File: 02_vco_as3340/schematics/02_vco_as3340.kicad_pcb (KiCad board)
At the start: 2 copper layers, 75 x 100 mm, 89 parts, among them J1 Header 1, J10 SINE OUT, J2 Header 2, J3 SYNC IN, J4 FM IN, J5 PWM CV IN, J6 1V per O IN, J7 SQUARE OUT, J8 SAW OUT, J9 TRI OUT, Q1 BC547C, Q2 BC547C, U1 TL072, U2 AS3340, U3 TL074

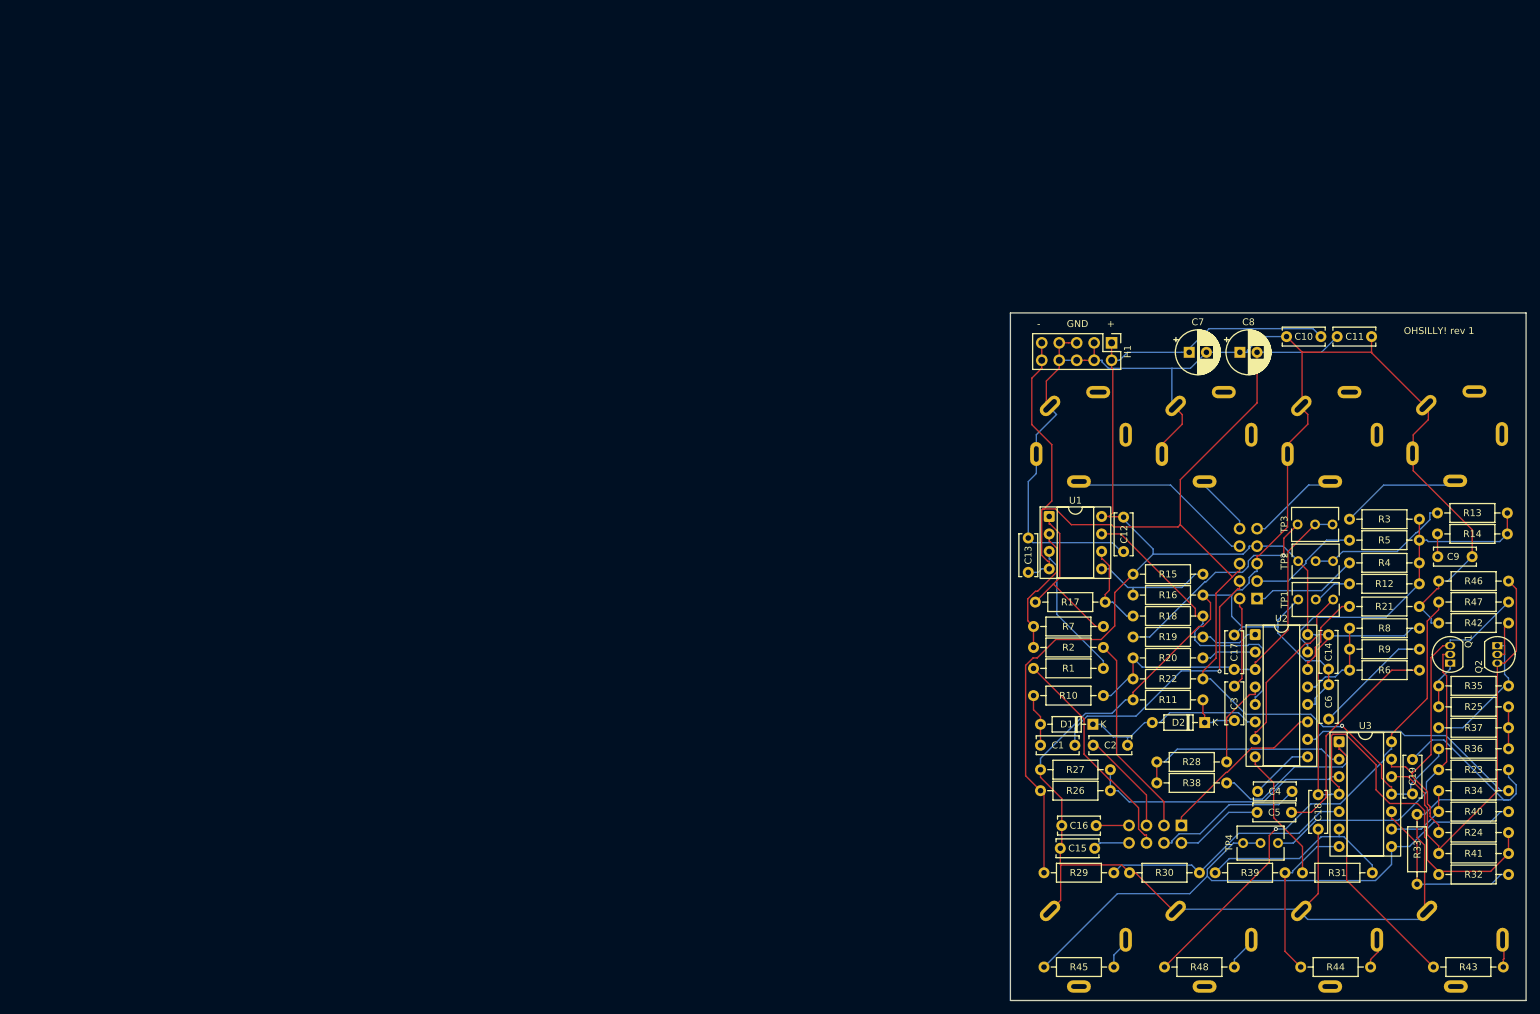
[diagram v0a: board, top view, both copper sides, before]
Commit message: 02 SMD!
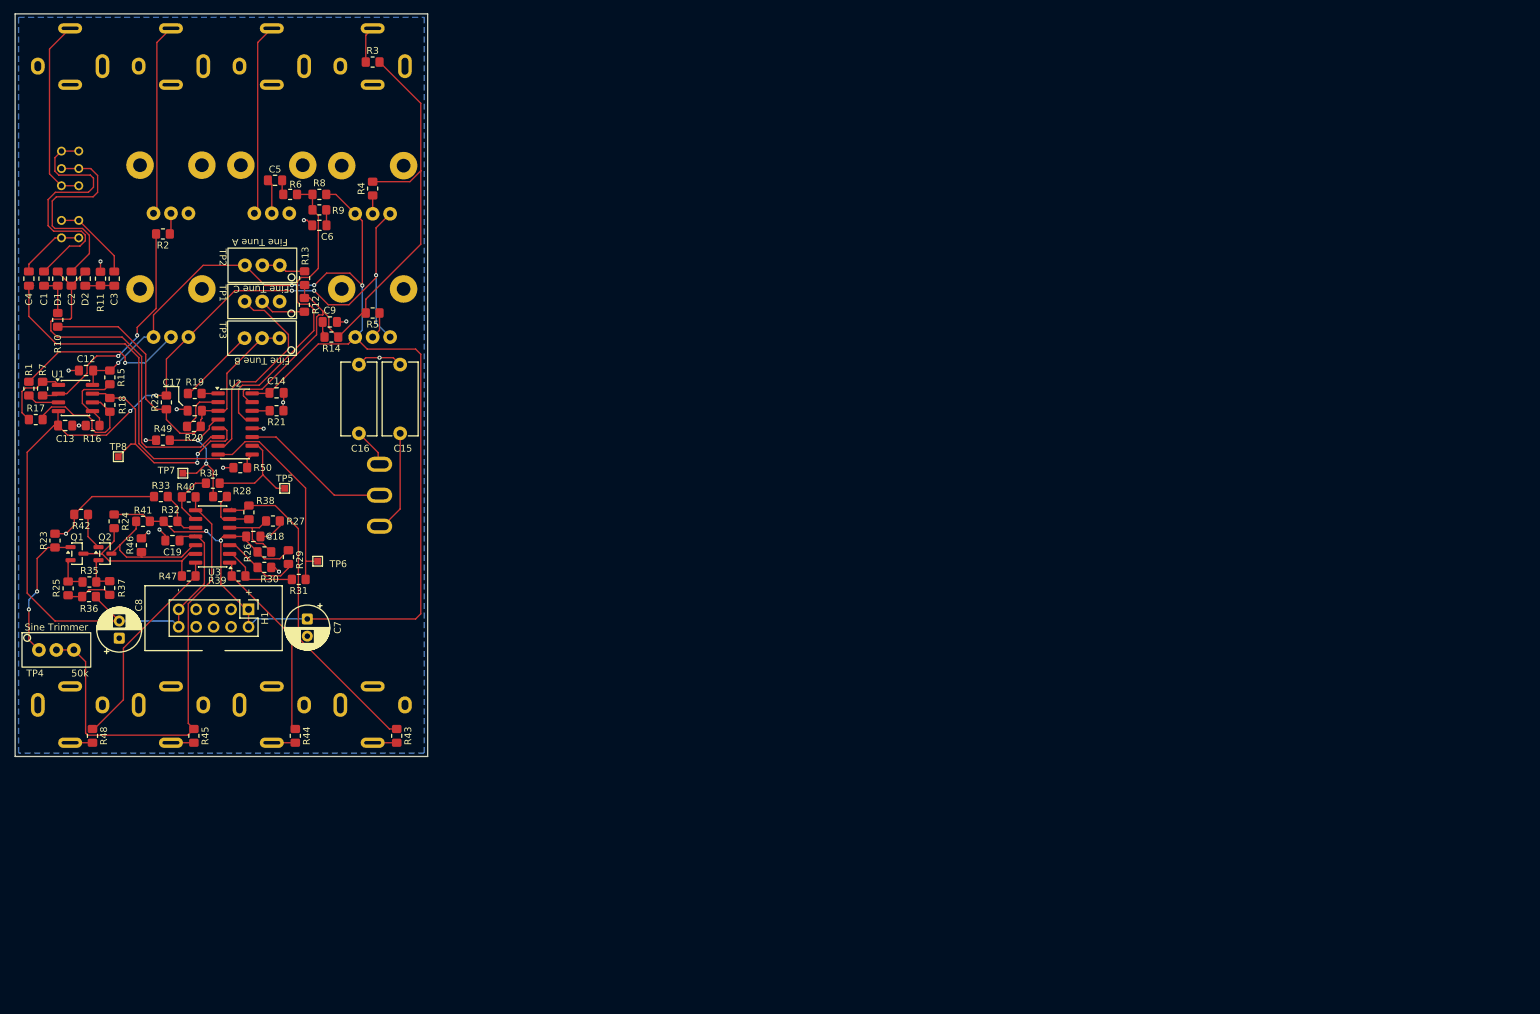
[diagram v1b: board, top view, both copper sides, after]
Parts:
- removed C10, C11: 100nF, Capacitor_THT:C_Disc_D6.0mm_W2.5mm_P5.00mm
- removed J1: Header 1, Connector_PinSocket_2.54mm:PinSocket_2x05_P2.54mm_Vertical
- removed J2: Header 2, Connector_PinSocket_2.54mm:PinSocket_2x04_P2.54mm_Vertical
- added R49: 51k, cynthia:R SMD 0805, F.Cu at (21.5, 62.0)
- added R50: 1M, cynthia:R SMD 0805, F.Cu at (32.8, 66.0)
- added RV1: 250k, cynthia:potientiometer, B.Cu at (22.7, 40.0)
- added RV2: 100k, cynthia:potientiometer, B.Cu at (37.3, 22.0)
- added RV3: 100k, cynthia:potientiometer, B.Cu at (22.7, 22.0)
- added RV4: 100k, cynthia:potientiometer, B.Cu at (52.0, 40.0)
- added RV5: 100k, cynthia:potientiometer, B.Cu at (52.0, 22.1)
- added SW1: ~, cynthia:switch_linear_1x4, B.Cu at (8.00, 27.0)
- added SW2: SW_SPDT, cynthia:switch, B.Cu at (53.0, 70.0)
- added TP5: TestPoint, TestPoint:TestPoint_Pad_1.0x1.0mm, F.Cu at (39.2, 69.0)
- added TP6: TestPoint, TestPoint:TestPoint_Pad_1.0x1.0mm, F.Cu at (44.0, 79.6)
- added TP7: TestPoint, TestPoint:TestPoint_Pad_1.0x1.0mm, F.Cu at (24.4, 66.8)
- added TP8: TestPoint, TestPoint:TestPoint_Pad_1.0x1.0mm, F.Cu at (15.0, 64.4)
- C1, C12, C13, C14, C17, C18, C19, C2, C3, C4, C5, C6, C9: footprint Capacitor_THT:C_Disc_D6.0mm_W2.5mm_P5.00mm -> cynthia:C SMD 0805
- C15, C16: footprint Capacitor_THT:C_Disc_D6.0mm_W2.5mm_P5.00mm -> Capacitor_THT:C_Disc_D10.5mm_W5.0mm_P10.00mm
- D1, D2: footprint Diode_THT:D_DO-35_SOD27_P7.62mm_Horizontal -> cynthia:C SMD 0805
- H1: footprint Connector_PinHeader_2.54mm:PinHeader_2x05_P2.54mm_Vertical -> cynthia:Eurorack Header
- J10, J7, J8, J9: footprint cynthia:6.35 mm jack socket mono in 3 pin socket tip pin west -> cynthia:3.5mm jack mono switched
- J3, J4, J5, J6: footprint cynthia:6.35 mm jack socket mono switched in 5 pin socket -> cynthia:3.5mm jack mono switched
- Q1, Q2: value BC547C -> BC847; footprint Package_TO_SOT_THT:TO-92_Inline -> Package_TO_SOT_SMD:SOT-23
- R1, R10, R11, R12, R13, R14, R15, R16, R17, R18, R19, R2, R20, R21, R22, R23, R24, R25, R26, R27, R28, R29, R3, R30, R31, R32, R33, R34, R35, R36, R37, R39, R4, R40, R41, R42, R43, R44, R45, R46, R47, R48, R5, R6, R7, R8, R9: footprint Resistor_THT:R_Axial_DIN0207_L6.3mm_D2.5mm_P10.16mm_Horizontal -> cynthia:R SMD 0805
- R38: value 82k -> 100k; footprint Resistor_THT:R_Axial_DIN0207_L6.3mm_D2.5mm_P10.16mm_Horizontal -> cynthia:R SMD 0805
- TP1, TP2, TP3, TP4: footprint Potentiometer_THT:Potentiometer_Vishay_T73XW_Horizontal -> cynthia:trimmer
- U1: footprint Package_DIP:DIP-8_W7.62mm_Socket -> cynthia:SOIC-8_3.9x4.9mm_P1.27mm
- U2: footprint Package_DIP:DIP-16_W7.62mm_Socket -> cynthia:SOIC-16_3.9x9.9mm_P1.27mm
- U3: footprint Package_DIP:DIP-14_W7.62mm_Socket -> cynthia:SOIC-14_3.9x8.7mm_P1.27mm
- moved R42 208.2 mm to (9.60, 72.8)
- moved R24 207.8 mm to (14.4, 73.8), turned to -90 degrees
- moved R36 207.6 mm to (10.8, 84.8), turned to 0 degrees
- moved R37 204.5 mm to (13.8, 83.5), turned to 90 degrees
- moved R41 204.4 mm to (18.6, 73.8)
- moved R23 204.0 mm to (5.80, 76.6), turned to 90 degrees
- moved Q2 203.0 mm to (13.1, 78.5), turned to 0 degrees
- moved Q1 200.4 mm to (9.00, 78.5), turned to 0 degrees
- moved R25 200.1 mm to (7.70, 83.6), turned to -90 degrees
- moved R46 198.9 mm to (18.4, 77.3), turned to 90 degrees
- moved R35 196.8 mm to (10.8, 82.6)
- moved C4 193.7 mm to (2.00, 38.5), turned to 90 degrees
- moved R47 192.0 mm to (25.2, 81.8), turned to 0 degrees
- moved R32 191.5 mm to (22.6, 73.8)
- moved R33 191.2 mm to (21.2, 70.2), turned to 180 degrees
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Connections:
- C1 pad 2: Hard Sync + -> Net-(C1-Pad2)
- C15 pad 1: Mode LFO -> GND
- C15 pad 2: GND -> Net-(SW2-A)
- C16 pad 1: GND -> Net-(SW2-C)
- C16 pad 2: Mode VCO -> GND
- C2 pad 2: Hard Sync -> Net-(C2-Pad2)
- C3 pad 2: Hard Sync - -> Net-(C3-Pad2)
- C4 pad 2: Soft Sync -> Net-(C4-Pad2)
- C5 pad 2: FM CV Levelled -> Net-(C5-Pad2)
- J3 pad T: Sync COM -> Net-(J3-PadT)
- J4 pad T: FM CV Hot -> Net-(J4-PadT)
- J5 pad T: PWM CV Hot -> Net-(J5-PadT)
- Q1 pad 1: Net-(Q1-E) -> Net-(Q1-B)
- Q1 pad 2: Net-(Q1-B) -> Net-(Q1-E)
- Q2 pad 1: Net-(Q2-E) -> Net-(Q2-B)
- Q2 pad 2: Net-(Q2-B) -> Net-(Q2-E)
- R1 pad 1: PWM Offset -> Net-(R1-Pad1)
- R2 pad 1: PWM CV Levelled -> Net-(R2-Pad1)
- R26 pad 2: Net-(U3A-+) -> Net-(U3B-+)
- R27 pad 1: Net-(U3A-+) -> Net-(U3B-+)
- R28 pad 2: Net-(U3A--) -> Net-(U3B--)
- R29 pad 2: Net-(U3B-+) -> Net-(U3A-+)
- R30 pad 1: Net-(U3B-+) -> Net-(U3A-+)
- R31 pad 2: Net-(U3B--) -> Net-(U3A--)
- R38 pad 1: Net-(U3A--) -> Net-(U3B--)
- R39 pad 1: Net-(U3B--) -> Net-(U3A--)
- R4 pad 1: Coarse Tuning -> Net-(R4-Pad1)
- R5 pad 1: Fine Tuning -> Net-(R5-Pad1)
- U2 pad 11: Mode COM -> Net-(SW2-B)
- U3 pad 1: Net-(R38-Pad2) -> Net-(R39-Pad2)
- U3 pad 7: Net-(R39-Pad2) -> Net-(R38-Pad2)
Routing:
- net GND: track 437.2 -> 49.6 mm, vias 0 -> 16
- net Net-(U2-VSSI): track 9.35 -> 55.8 mm
- net +12V: track 260.0 -> 214.3 mm, vias 0 -> 6
- net Net-(R47-Pad2): track 73.0 -> 30.5 mm, vias 1 -> 0
- net Hard Sync +: track 41.5 -> 0.00 mm, vias 1 -> 0
- net Net-(Q2-C): track 60.3 -> 19.8 mm
- net Net-(C1-Pad2): track 0.00 -> 39.0 mm
- net Net-(U2-VFCI): track 49.6 -> 86.0 mm
- net Net-(U2-VLFI): track 13.2 -> 46.4 mm
- net PWM Offset: track 32.4 -> 0.00 mm
- net Net-(C2-Pad2): track 0.00 -> 31.2 mm
- net Net-(C5-Pad1): track 32.4 -> 2.12 mm
- net PWM CV Levelled: track 29.5 -> 0.00 mm
- net Net-(J4-PadT): track 0.00 -> 28.0 mm
- net Net-(J5-PadT): track 0.00 -> 28.0 mm
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- added copper zone on B.Cu, net GND
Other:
- board size 75 x 100 mm -> 60 x 108 mm
- board text removed: "+"
- board text removed: "-"
- board text removed: "GND"
- board text removed: "OHSILLY! rev 1"
